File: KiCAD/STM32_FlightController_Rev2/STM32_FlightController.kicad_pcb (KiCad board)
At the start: 4 copper layers, 42 x 44.4 mm, 56 parts, among them J1 629105150521, J2 JST_SH_SM08B-SRSS-TB_1x08-1MP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, J3 JST_SH_SM04B-SRSS-TB_1x04-1MP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, J4 JST_SH_SM04B-SRSS-TB_1x04-1MP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, J5 Conn_02x05_Odd_Even, SW1 PTS815SJM250SMTRLFS, SW2 PCM12SMTR, U1 SN74LVC1T45DBV, U2 ICM-20948, U3 STM32F405RGTx, U4 USBLC6-2SC6, U5 AMS1117-3.3, U6 TLV70018, U7 BMP390L, U8 SN74LVC1T45DBV, Y1 X32258MOB4SI

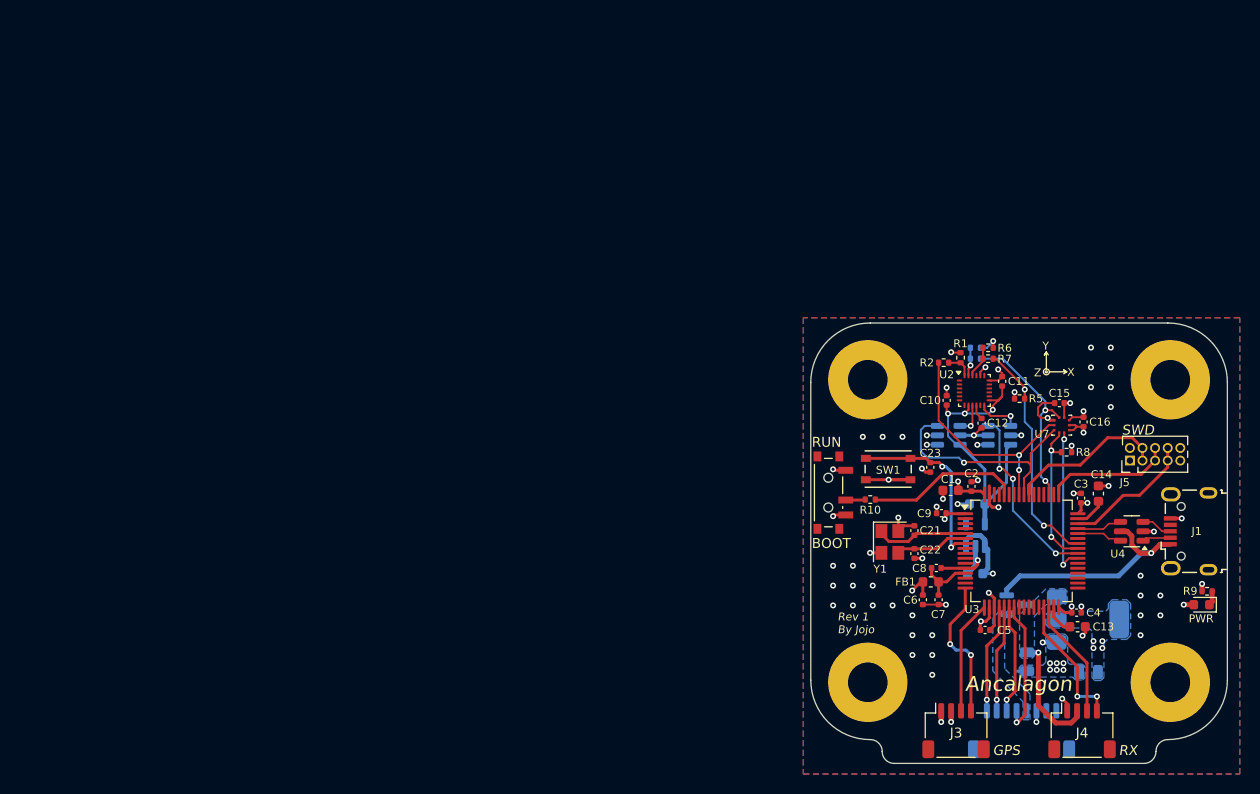
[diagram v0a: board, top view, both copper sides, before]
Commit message: added manufacturing related files
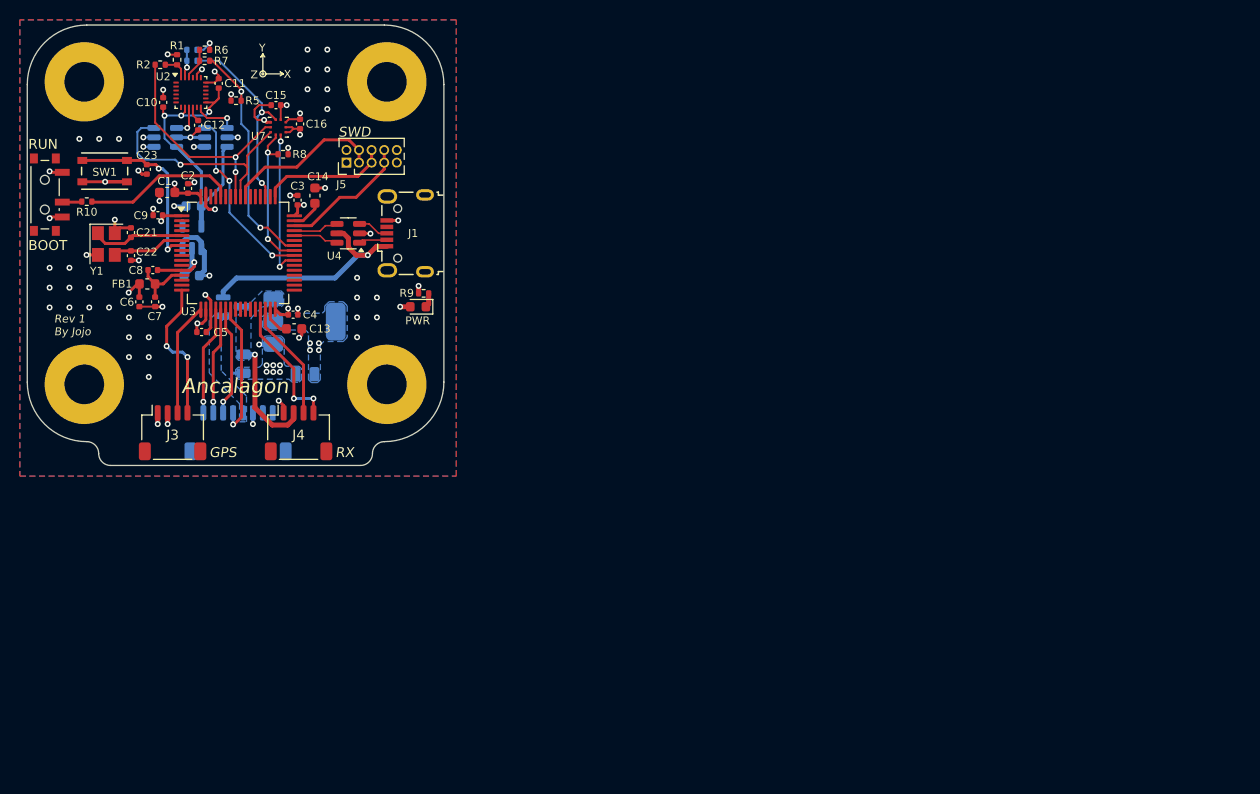
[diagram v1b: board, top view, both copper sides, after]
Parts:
- moved C13 84.5 mm to (41.7, 45.1)
- moved C7 84.5 mm to (27.6, 42.4)
- moved J1 84.5 mm to (52.9, 35.5)
- moved C10 84.5 mm to (28.5, 22.3)
- moved C11 84.5 mm to (34.1, 20.4)
- moved C12 84.5 mm to (32.0, 24.6)
- moved C14 84.5 mm to (43.8, 31.7)
- moved C16 84.5 mm to (42.3, 24.5)
- moved C17 84.5 mm to (31.3, 39.8)
- moved C18 84.5 mm to (31.5, 32.7)
- moved C2 84.5 mm to (31.0, 31.0)
- moved C21 84.5 mm to (25.2, 35.4)
- moved C22 84.5 mm to (25.2, 37.7)
- moved C23 84.5 mm to (26.8, 29.0)
- moved C3 84.5 mm to (42.0, 32.1)
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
